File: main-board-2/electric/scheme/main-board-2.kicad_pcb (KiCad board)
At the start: 2 copper layers, 85 x 56 mm, 122 parts, among them K1 power-switch, K2 usb-power-switch, P1 batt, P10 rst, P11 screw-1, P13 screw-2, P14 gpio-big, P15 gpio-small, P16 moto-1, P17 moto-2, P3 trigger-btn, P4 CONN_3X2, P7 bootloader, P8 cross board conn, P9 rst, Q1 IRLML2244, Q10 IRLML2244, Q11 sot223, Q12 bc857, Q13 irlml2244, Q2 BC847, Q3 IRLML2244, Q4 IRLML2244, Q5 BC847, Q6 BC847, Q7 BC847, Q8 BC847, Q9 IRLML2244, U1 LM317AEMP, U2 LM317AT, U3 LM317AEMP, U4 LM317AT, U5 LM293, U6 L298, U7 MINI-USB-B, X1 8MHz

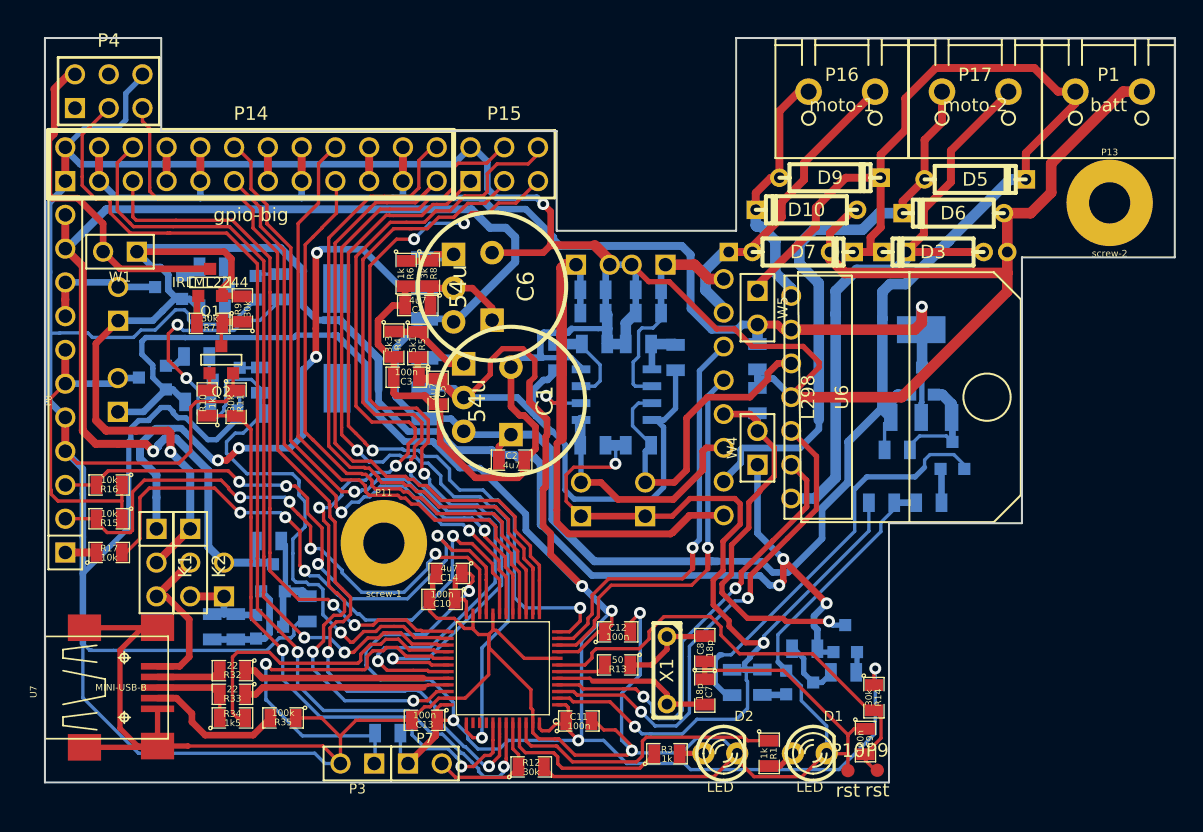
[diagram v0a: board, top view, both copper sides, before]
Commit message: Added comments.
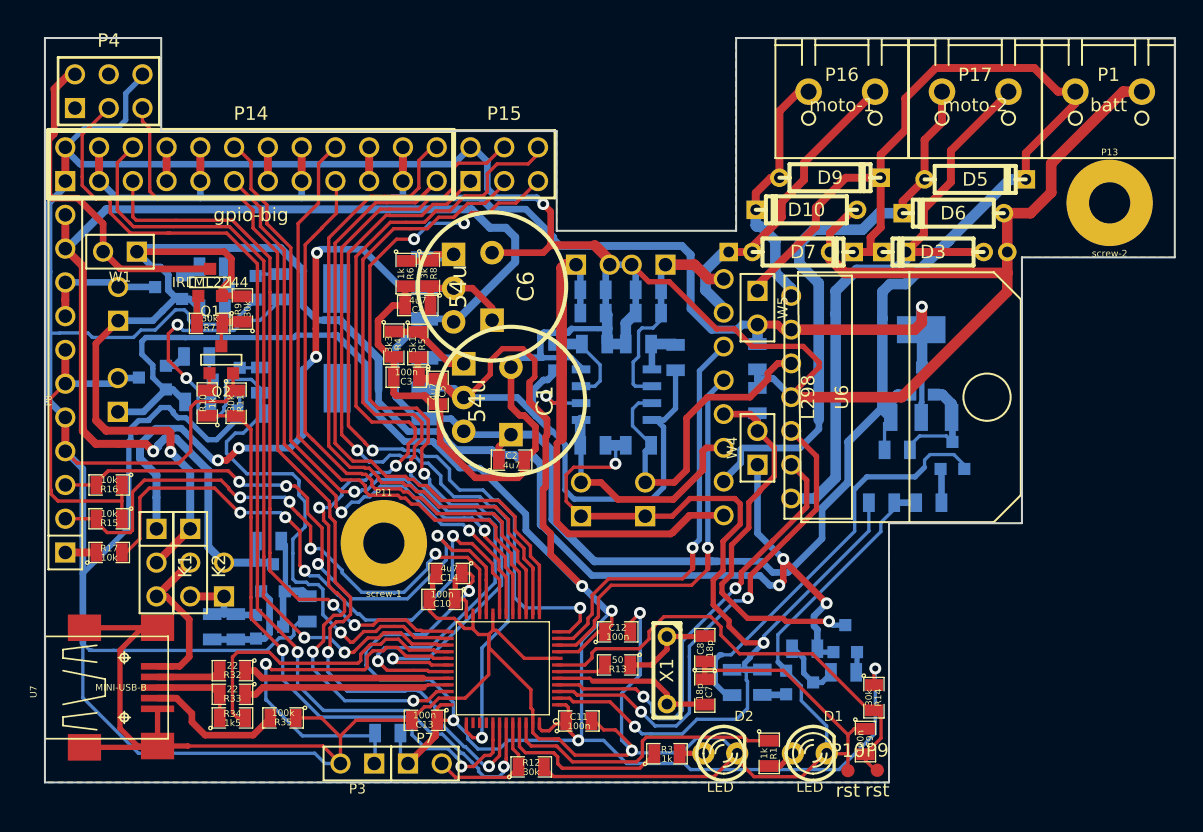
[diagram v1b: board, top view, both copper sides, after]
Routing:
- added copper zone on B.Cu, net GND
- added copper zone on F.Cu, net GND
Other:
- board text added: "+ -"
- board text added: "1"
- board text added: "2"
- board text added: "3"
- board text added: "4"
- board text added: "5,1"
- board text added: "6,2"
- board text added: "7,3"
- board text added: "8,4"
- board text added: "V"
- board text added: "boot loader"
- board text added: "c,rx"
- board text added: "d,tx"
- board text added: "gnd"
- board text added: "gnd,9"
- board text added: "moto 1, 2, 3, 4"
- board text added: "pwr routing"
- board text added: "rst"
- board text added: "trigger"
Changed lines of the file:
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@@
     (area 127.606667 112.000001 242.964763 190.8)
     (thickness 1.6)
-    (drawings 57)
+    (drawings 84)
     (tracks 2008)
     (zones 0)
@@
     (pad_to_mask_clearance 0)
     (aux_axis_origin 143.5 181)
-    (visible_elements 7FFFFBFF)
+    (visible_elements 7FFFFFFF)
     (pcbplotparams
       (layerselection 3178497)
@@
     )
   )
+  (gr_text "pwr\nrouting" (at 155.5 158.5) (layer Cmts.User)
+    (effects (font (size 2 2) (thickness 0.3)) (justify left))
+  )
+  (gr_text 4 (at 158.25 165.75) (layer Cmts.User)
+    (effects (font (size 2 2) (thickness 0.3)))
+  )
+  (gr_text 3 (at 154.5 159.5) (layer Cmts.User)
+    (effects (font (size 2 2) (thickness 0.3)))
+  )
+  (gr_text 2 (at 151.5 159.5) (layer Cmts.User)
+    (effects (font (size 2 2) (thickness 0.3)))
+  )
+  (gr_text 1 (at 149.75 166.75) (layer Cmts.User)
+    (effects (font (size 2 2) (thickness 0.3)))
+  )
+  (gr_text gnd,9 (at 175.5 138.5 90) (layer Eco2.User)
+    (effects (font (size 1 1) (thickness 0.25)) (justify mirror))
+  )
+  (gr_text 8,4 (at 173 138.75 90) (layer Eco2.User)
+    (effects (font (size 1.5 1.5) (thickness 0.3)) (justify mirror))
+  )
+  (gr_text 7,3 (at 165.5 138.75 90) (layer Eco2.User)
+    (effects (font (size 1.5 1.5) (thickness 0.3)) (justify mirror))
+  )
+  (gr_text 6,2 (at 157.75 138.75 90) (layer Eco2.User)
+    (effects (font (size 1.5 1.5) (thickness 0.3)) (justify mirror))
+  )
+  (gr_text 5,1 (at 150.25 138.75 90) (layer Eco2.User)
+    (effects (font (size 1.5 1.5) (thickness 0.3)) (justify mirror))
+  )
+  (gr_text d,tx (at 180.5 138.75 90) (layer Eco2.User)
+    (effects (font (size 1.5 1.5) (thickness 0.3)) (justify mirror))
+  )
+  (gr_text c,rx (at 178 138.75 90) (layer Eco2.User)
+    (effects (font (size 1.5 1.5) (thickness 0.3)) (justify mirror))
+  )
+  (gr_text gnd (at 168 138.75 90) (layer Eco2.User)
+    (effects (font (size 1.5 1.5) (thickness 0.3)) (justify mirror))
+  )
+  (gr_text gnd (at 160.25 138.75 90) (layer Eco2.User)
+    (effects (font (size 1.5 1.5) (thickness 0.3)) (justify mirror))
+  )
+  (gr_text gnd (at 152.75 138.75 90) (layer Eco2.User)
+    (effects (font (size 1.5 1.5) (thickness 0.3)) (justify mirror))
+  )
+  (gr_text V (at 170.5 138.75 90) (layer Eco2.User)
+    (effects (font (size 2 2) (thickness 0.3)) (justify mirror))
+  )
+  (gr_text V (at 162.75 138.75 90) (layer Eco2.User)
+    (effects (font (size 2 2) (thickness 0.3)) (justify mirror))
+  )
+  (gr_text V (at 155.5 138.75 90) (layer Eco2.User)
+    (effects (font (size 2 2) (thickness 0.3)) (justify mirror))
+  )
+  (gr_text V (at 147.5 138.75 90) (layer Eco2.User)
+    (effects (font (size 2 2) (thickness 0.3)) (justify mirror))
+  )
+  (gr_text "boot\nloader" (at 170 172.5 90) (layer Eco2.User)
+    (effects (font (size 1.5 1.5) (thickness 0.3)) (justify mirror))
+  )
+  (gr_text trigger (at 166.75 173.5 90) (layer Eco2.User)
+    (effects (font (size 1.5 1.5) (thickness 0.3)) (justify mirror))
+  )
+  (gr_text "moto 1, 2, 3, 4" (at 208.25 132.5) (layer Eco2.User)
+    (effects (font (size 1.5 1.5) (thickness 0.3)) (justify mirror))
+  )
+  (gr_text "+ -" (at 223.5 133.5) (layer Eco2.User)
+    (effects (font (size 3 3) (thickness 0.3)))
+  )
+  (gr_text "boot\nloader" (at 169.75 172 90) (layer Cmts.User)
+    (effects (font (size 1.5 1.5) (thickness 0.3)))
+  )
+  (gr_text trigger (at 166.75 172.75 90) (layer Cmts.User)
+    (effects (font (size 1.5 1.5) (thickness 0.3)))
+  )
+  (gr_text rst (at 203.75 176.5 90) (layer Cmts.User)
+    (effects (font (size 1.5 1.5) (thickness 0.3)))
+  )
+  (gr_text "+ -" (at 223.5 133.5) (layer Cmts.User)
+    (effects (font (size 3 3) (thickness 0.3)))
+  )
   (gr_circle (center 160.655 153.67) (end 162.179 153.8478) (layer Dwgs.User) (width 0.2))
   (gr_circle (center 160.7312 143.2052) (end 162.2552 143.4338) (layer Dwgs.User) (width 0.2))
@@
   (segment (start 153.64206 172.26534) (end 154.3558 171.5516) (width 0.5) (layer F.Cu) (net 45))
   (segment (start 151.892 167.005) (end 154.432 164.465) (width 0.6) (layer F.Cu) (net 45))
-  (segment (start 179.56022 156.75356) (end 179.56022 157.62478) (width 0.5) (layer F.Cu) (net 46) (status 400000))
+  (segment (start 179.56022 156.75356) (end 179.56022 157.62478) (width 0.5) (layer F.Cu) (net 46))
   (segment (start 173.228 155.42768) (end 173.228 154.7876) (width 0.5) (layer F.Cu) (net 46))
   (segment (start 175.88484 158.08452) (end 173.228 155.42768) (width 0.5) (layer F.Cu) (net 46))
   (segment (start 179.10048 158.08452) (end 175.88484 158.08452) (width 0.5) (layer F.Cu) (net 46))
   (segment (start 179.56022 157.62478) (end 179.10048 158.08452) (width 0.5) (layer F.Cu) (net 46))
-  (segment (start 173.228 154.7876) (end 173.228 152.68702) (width 0.5) (layer F.Cu) (net 46) (status 800000))
-  (segment (start 173.228 152.68702) (end 173.08068 152.5397) (width 0.5) (layer F.Cu) (net 46) (status C00000))
+  (segment (start 173.228 154.7876) (end 173.228 152.68702) (width 0.5) (layer F.Cu) (net 46))
+  (segment (start 173.228 152.68702) (end 173.08068 152.5397) (width 0.5) (layer F.Cu) (net 46))
   (segment (start 173.08068 152.5397) (end 172.6819 152.5397) (width 0.6) (layer F.Cu) (net 46))
   (segment (start 172.6819 152.5397) (end 172.0596 151.9174) (width 0.6) (layer F.Cu) (net 46))
@@
   (segment (start 183.61914 171.16806) (end 185.1152 169.672) (width 0.254) (layer F.Cu) (net 83))
   (segment (start 185.1152 169.672) (end 185.6359 169.672) (width 0.254) (layer F.Cu) (net 83))
+  (zone (net 46) (net_name GND) (layer F.Cu) (hatch edge 0.508)
+    (connect_pads (clearance 0.508))
+    (min_thickness 0.254)
+    (fill (arc_segments 16) (thermal_gap 0.508) (thermal_bridge_width 0.508))
+    (polygon
+      (pts
+        (xy 228.5 141.5) (xy 217 141.5) (xy 217 161.5) (xy 207 161.5) (xy 207 181)
+        (xy 143.5 181) (xy 143.5 125) (xy 152.25 125) (xy 152.25 132) (xy 182 132)
+        (xy 182 139.5) (xy 195.5 139.5) (xy 195.5 125) (xy 228.5 125)
+      )
+    )
+  )
+  (zone (net 46) (net_name GND) (layer B.Cu) (hatch edge 0.508)
+    (connect_pads (clearance 0.508))
+    (min_thickness 0.254)
+    (fill (arc_segments 16) (thermal_gap 0.508) (thermal_bridge_width 0.508))
+    (polygon
+      (pts
+        (xy 228.5 141.5) (xy 217 141.5) (xy 217 161.5) (xy 207 161.5) (xy 207 181)
+        (xy 143.5 181) (xy 143.5 125) (xy 152.25 125) (xy 152.25 132) (xy 182 132)
+        (xy 182 139.5) (xy 195.5 139.5) (xy 195.5 125) (xy 228.5 125)
+      )
+    )
+  )
 )
